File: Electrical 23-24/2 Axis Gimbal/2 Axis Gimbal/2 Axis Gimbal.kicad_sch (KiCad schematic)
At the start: 25 parts, among them IC1 BNO085, J1 Conn_01x06_Socket, U1 ATtiny404-SS

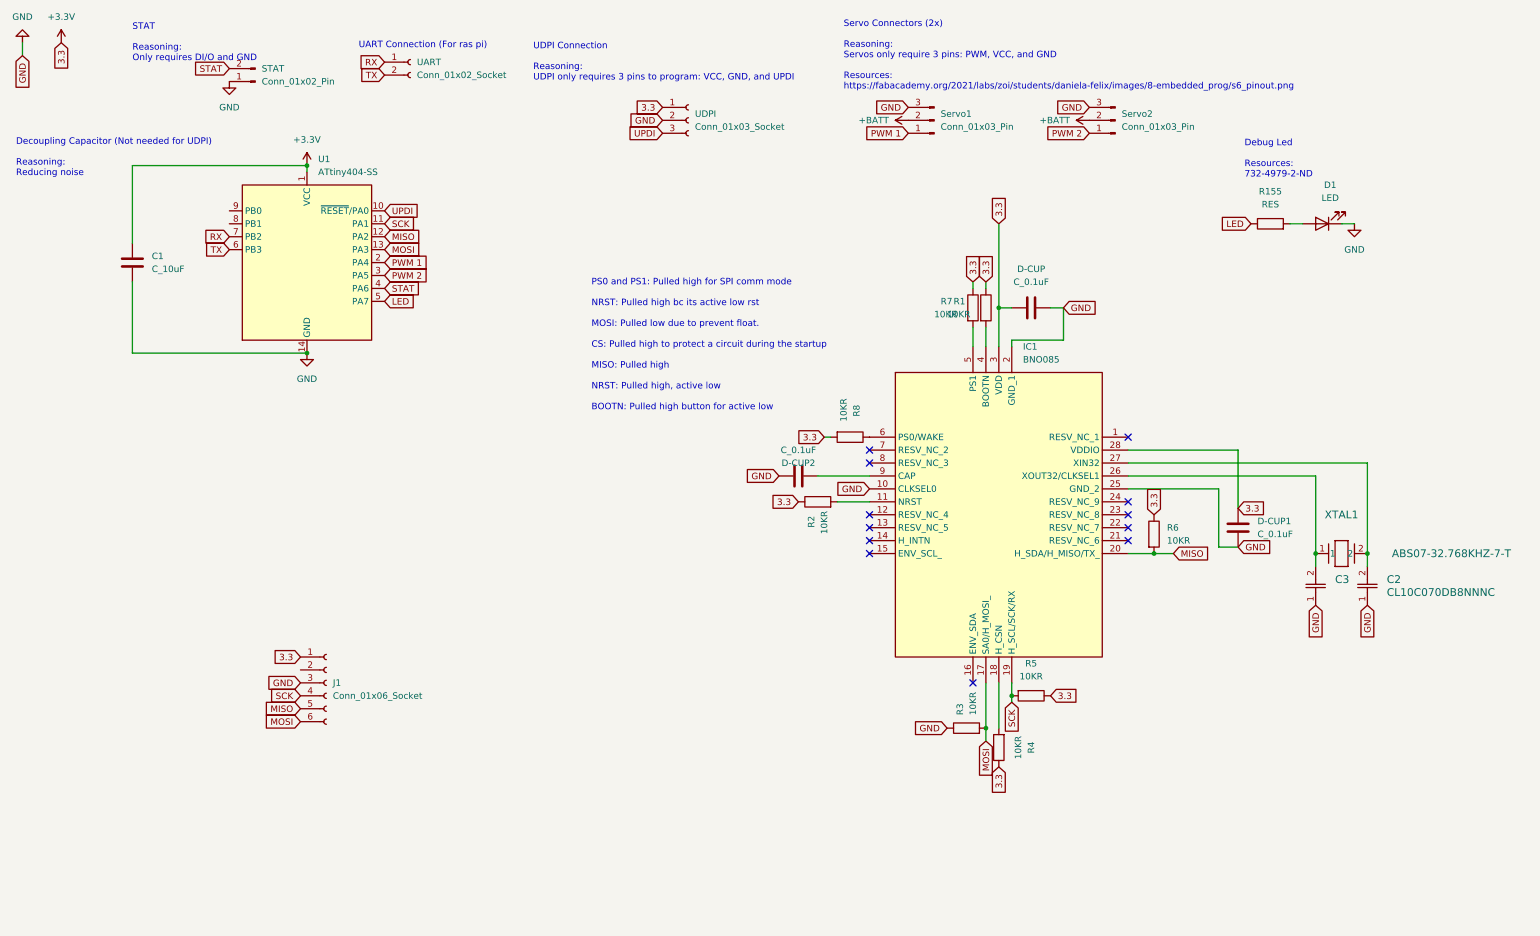
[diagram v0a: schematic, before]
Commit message: Fix some gimbal problems
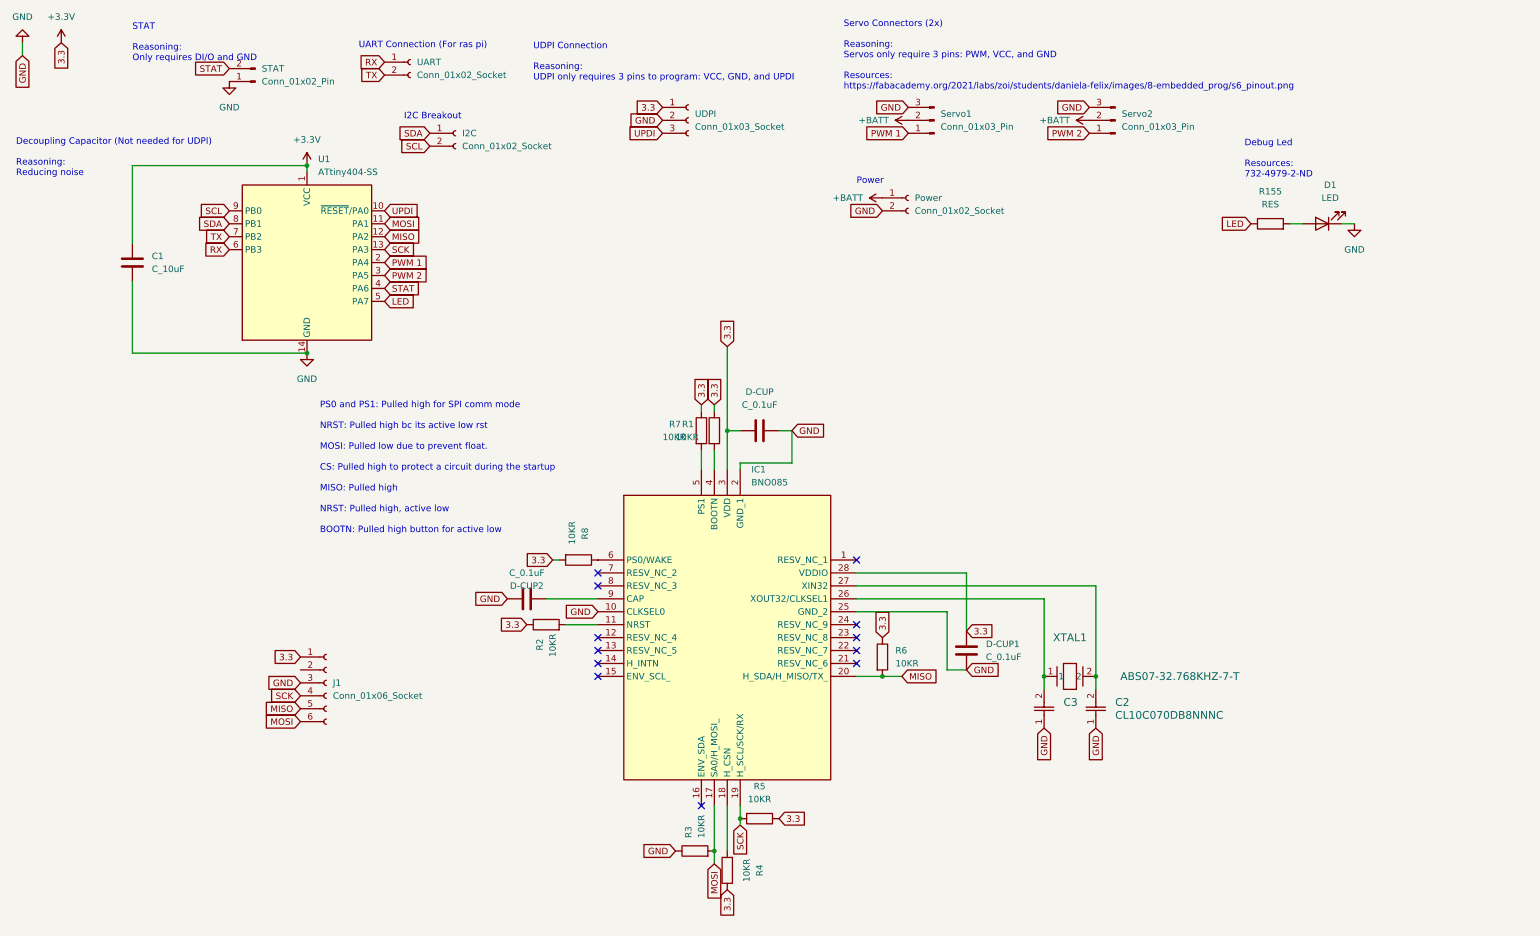
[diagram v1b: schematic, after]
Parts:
- added I2C, Power: Conn_01x02_Socket, symbol Connector:Conn_01x02_Socket
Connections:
- net +BATT: now also Power.1 (Pin_1)
- net GND: now also Power.2 (Pin_2)
- net MOSI: now also U1.11 (PA1); no longer U1.13 (PA3)
- net RX: now also U1.6 (PB3); no longer U1.7 (PB2)
- net SCK: now also U1.13 (PA3); no longer U1.11 (PA1)
- net TX: now also U1.7 (PB2); no longer U1.6 (PB3)
- net SDA: now reaches U1.8 (PB1)
- net SDA: now also I2C.1 (Pin_1)
- net SCL: now reaches U1.9 (PB0)
- net SCL: now also I2C.2 (Pin_2)
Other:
- note added: "I2C Breakout"
- note added: "Power"
- moved on the sheet: C2, C3, D-CUP, D-CUP1, D-CUP2, IC1, R1, R2, R3, R4, R5, R6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
